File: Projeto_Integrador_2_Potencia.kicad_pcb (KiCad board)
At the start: 2 copper layers, 101 x 59.2 mm, 18 parts, among them J10 Borne_CMD_Interface, J2 Vi 24V, J3 Vo 48V, J4 INA219_01x02_Socket_3.5mm, J5 INA219_01x06_Socket_2.55mm, J7 Display_01x04_Socket, J9 JST_01x02_Pin, Q1 IRF740

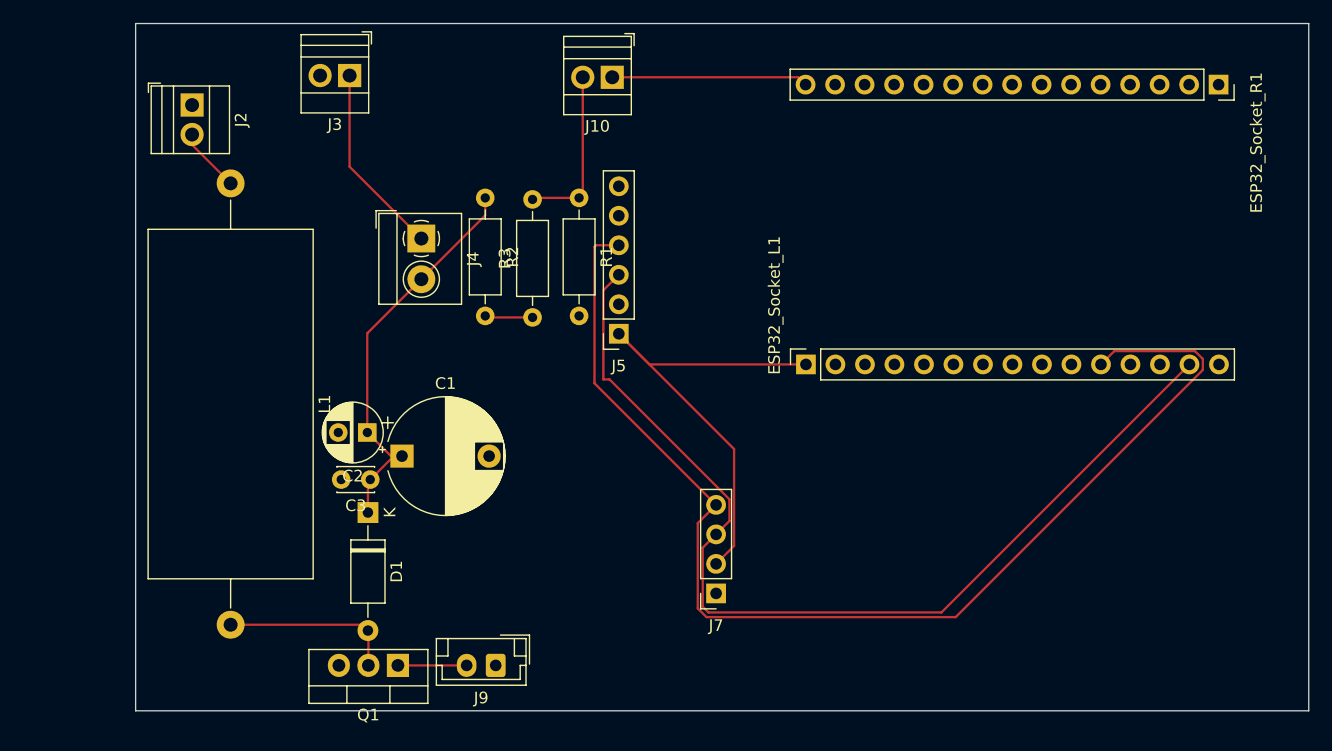
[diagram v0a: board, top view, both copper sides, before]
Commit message: Adição de footprint e símbolo do ESP32
Atualização das trilhas da PCB
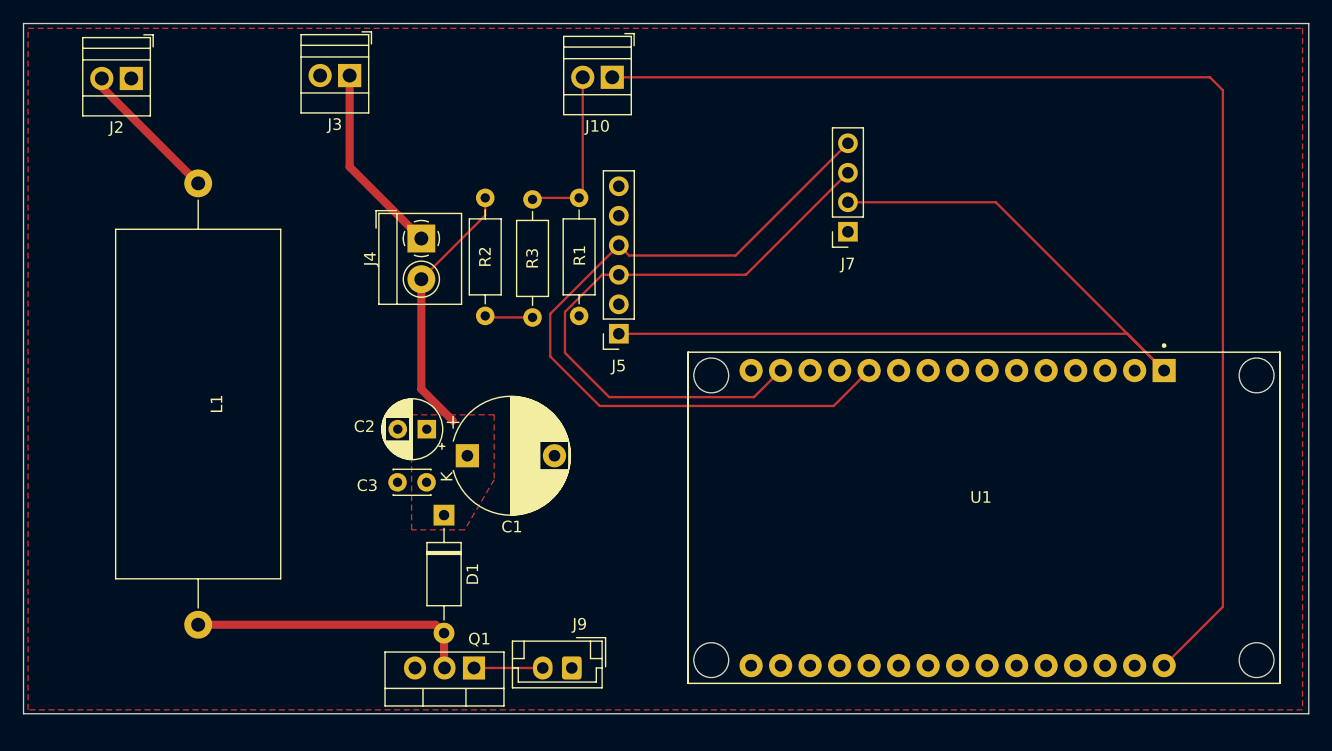
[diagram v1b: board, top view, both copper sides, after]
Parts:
- removed ESP32_Socket_L1, ESP32_Socket_R1: ~, Connector_PinSocket_2.54mm:PinSocket_1x15_P2.54mm_Vertical
- added U1: ESP32-DEVKIT-V1, footprints_and_symbols:MODULE_ESP32_DEVKIT_V1, F.Cu at (165.4, 88.6)
- J9: value JST_01x02_Pin -> PWM_Connector
- moved J7 33.1 mm to (153.6, 64.0)
- moved J9 6.56 mm to (129.9, 101.6)
- moved D1 6.56 mm to (118.9, 88.4)
- moved Q1 6.56 mm to (121.5, 101.6)
- moved J2 5.71 mm to (91.9, 50.8), turned to 180 degrees
- moved C1 5.63 mm to (120.9, 83.3)
- moved C2 5.13 mm to (117.4, 81.0)
- moved C3 4.85 mm to (117.4, 85.6)
- moved L1 2.79 mm to (97.7, 59.8)
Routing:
- net 12V: track 16.9 -> 104.7 mm
- net 3V3: track 41.8 -> 81.5 mm
- net I2C_Sda: track 101.4 -> 66.6 mm
- net I2C_Scl: track 85.8 -> 53.9 mm
- net INA_Vin-: track 34.7 -> 22.6 mm
- net Net-(D1-A): track 15.8 -> 26.0 mm
- net Net-(J2-Pin_2): track 5.58 -> 12.5 mm
- added copper zone on F.Cu, net GND
- added copper zone on F.Cu, net INA_Vin-
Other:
- board size 101 x 59.2 mm -> 110.7 x 59.4 mm
- board text removed: "ESP32 DevKitV1 30P"
